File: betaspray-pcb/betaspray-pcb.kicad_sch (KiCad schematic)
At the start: 1 part, among them U1 ESP32-S3

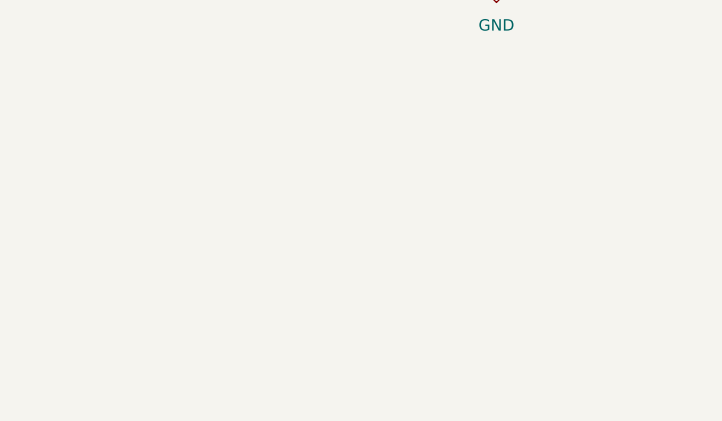
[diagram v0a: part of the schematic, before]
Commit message: Add LDO
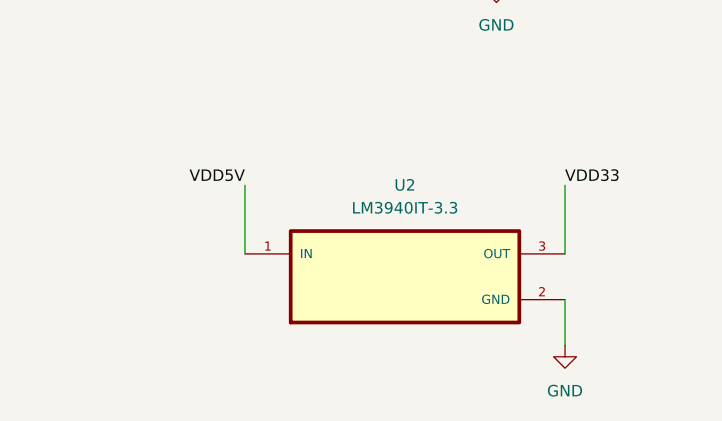
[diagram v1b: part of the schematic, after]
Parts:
- added U2: LM3940IT-3.3, LM3940IT-3.3:TO254P1054X470X1955-3, symbol betaspray_LDO:LM3940IT-3.3
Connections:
- net GND: now also U2.2 (GND)
- new net VDD33: U2.3 (OUT)
- new net VDD5V: U2.1 (IN)
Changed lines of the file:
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@@
+		)
+	)
+	(wire
+		(pts
+			(xy 74.93 143.51) (xy 74.93 151.13)
+		)
+		(stroke
+			(width 0)
+			(type default)
+		)
+	)
+	(wire
+		(pts
+			(xy 110.49 143.51) (xy 110.49 151.13)
+		)
+		(stroke
+			(width 0)
+			(type default)
+		)
+	)
+	(wire
+		(pts
+			(xy 110.49 156.21) (xy 110.49 161.29)
+		)
+		(stroke
+			(width 0)
+			(type default)
+		)
+	)
+	(label "VDD33"
+		(at 110.49 143.51 0)
+		(effects
+			(font
+				(size 1.27 1.27)
+			)
+			(justify left bottom)
+		)
+	)
+	(label "VDD5V"
+		(at 74.93 143.51 180)
+		(effects
+			(font
+				(size 1.27 1.27)
+			)
+			(justify right bottom)
+		)
+	)
+	(symbol
+		(lib_id "betaspray_LDO:LM3940IT-3.3")
+		(at 92.71 153.67 0)
+		(unit 1)
+		(exclude_from_sim no)
+		(in_bom yes)
+		(on_board yes)
+		(dnp no)
+		(fields_autoplaced yes)
+		(property "Reference" "U2"
+			(at 92.71 143.51 0)
+			(effects
+				(font
+					(size 1.27 1.27)
+				)
+			)
+		)
+		(property "Value" "LM3940IT-3.3"
+			(at 92.71 146.05 0)
+			(effects
+				(font
+					(size 1.27 1.27)
+				)
+			)
+		)
+		(property "Footprint" "LM3940IT-3.3:TO254P1054X470X1955-3"
+			(at 92.71 153.67 0)
+			(effects
+				(font
+					(size 1.27 1.27)
+				)
+				(justify bottom)
+				(hide yes)
+			)
+		)
+		(property "Datasheet" ""
+			(at 92.71 153.67 0)
+			(effects
+				(font
+					(size 1.27 1.27)
+				)
+				(hide yes)
+			)
+		)
+		(property "Description" ""
+			(at 92.71 153.67 0)
+			(effects
+				(font
+					(size 1.27 1.27)
+				)
+				(hide yes)
+			)
+		)
+		(pin "3"
+		)
+		(pin "2"
+		)
+		(pin "1"
+		)
+		(instances
+			(project ""
+				(path "/5d34c70f-469d-43be-b671-484e3b695429"
+					(reference "U2")
+					(unit 1)
+				)
+			)
 		)
 	)
 	(symbol
 		(lib_id "power:GND")
+		(at 110.49 161.29 0)
+		(unit 1)
+		(exclude_from_sim no)
+		(in_bom yes)
+		(on_board yes)
+		(dnp no)
+		(fields_autoplaced yes)
+		(property "Reference" "#PWR02"
+			(at 110.49 167.64 0)
+			(effects
+				(font
+					(size 1.27 1.27)
+				)
+				(hide yes)
+			)
+		)
+		(property "Value" "GND"
+			(at 110.49 166.37 0)
+			(effects
+				(font
+					(size 1.27 1.27)
+				)
+			)
+		)
+		(property "Footprint" ""
+			(at 110.49 161.29 0)
+			(effects
+				(font
+					(size 1.27 1.27)
+				)
+				(hide yes)
+			)
+		)
+		(property "Datasheet" ""
+			(at 110.49 161.29 0)
+			(effects
+				(font
+					(size 1.27 1.27)
+				)
+				(hide yes)
+			)
+		)
+		(property "Description" "Power symbol creates a global label with name \"GND\" , ground"
+			(at 110.49 161.29 0)
+			(effects
+				(font
+					(size 1.27 1.27)
+				)
+				(hide yes)
+			)
+		)
+		(pin "1"
+		)
+		(instances
+			(project ""
+				(path "/5d34c70f-469d-43be-b671-484e3b695429"
+					(reference "#PWR02")
+					(unit 1)
+				)
+			)
+		)
+	)
+	(symbol
+		(lib_id "power:GND")
